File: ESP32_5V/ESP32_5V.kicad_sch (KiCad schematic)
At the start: 4 parts

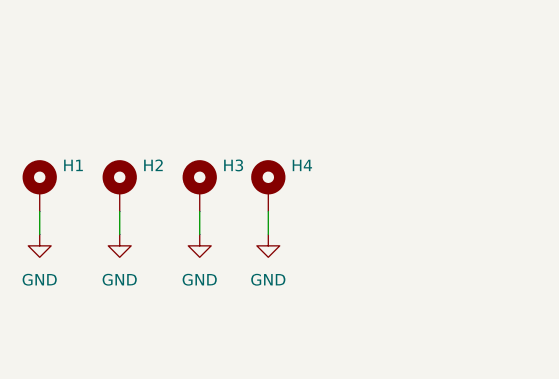
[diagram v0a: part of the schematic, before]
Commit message: update
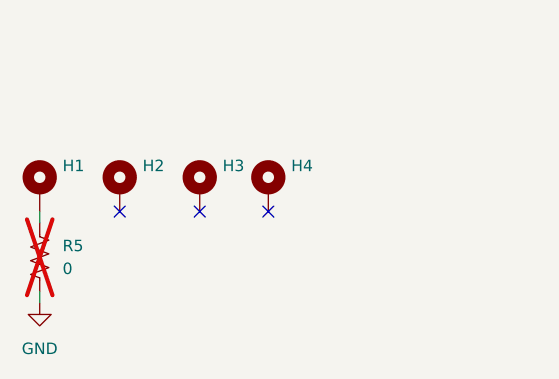
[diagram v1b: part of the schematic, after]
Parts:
- added R5: 0, symbol Device:R_US
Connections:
- net GND: now also R5.2; no longer H1.1, H2.1, H3.1, H4.1
- new net: H1.1, R5.1
- no-connect marks 0 -> 3
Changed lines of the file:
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@@
 		(color 0 0 0 0)
 	)
+	(no_connect
+		(at 57.15 177.8)
+	)
+	(no_connect
+		(at 40.64 177.8)
+	)
+	(no_connect
+		(at 49.53 177.8)
+	)
 	(wire
 		(pts
@@
 	(wire
 		(pts
-			(xy 31.75 180.34) (xy 31.75 177.8)
-		)
-		(stroke
-			(width 0)
-			(type default)
-		)
-	)
-	(wire
-		(pts
 			(xy 175.26 82.55) (xy 175.26 64.77)
 		)
@@
 	(wire
 		(pts
-			(xy 40.64 180.34) (xy 40.64 177.8)
-		)
-		(stroke
-			(width 0)
-			(type default)
-		)
-	)
-	(wire
-		(pts
 			(xy 185.42 127.635) (xy 185.42 62.23)
 		)
@@
 	(wire
 		(pts
+			(xy 31.75 187.96) (xy 31.75 186.69)
+		)
+		(stroke
+			(width 0)
+			(type default)
+		)
+	)
+	(wire
+		(pts
 			(xy 176.53 80.01) (xy 176.53 62.23)
 		)
@@
 	(wire
 		(pts
-			(xy 49.53 180.34) (xy 49.53 177.8)
-		)
-		(stroke
-			(width 0)
-			(type default)
-		)
-	)
-	(wire
-		(pts
 			(xy 139.065 97.155) (xy 170.18 97.155)
 		)
@@
 	(wire
 		(pts
-			(xy 57.15 180.34) (xy 57.15 177.8)
-		)
-		(stroke
-			(width 0)
-			(type default)
-		)
-	)
-	(wire
-		(pts
 			(xy 185.42 62.23) (xy 185.42 44.45)
 		)
@@
 		(pts
 			(xy 189.23 54.61) (xy 204.47 54.61)
+		)
+		(stroke
+			(width 0)
+			(type default)
+		)
+	)
+	(wire
+		(pts
+			(xy 31.75 179.07) (xy 31.75 177.8)
 		)
 		(stroke
@@
 	(symbol
 		(lib_id "power:GND")
-		(at 49.53 180.34 0)
-		(unit 1)
-		(exclude_from_sim no)
-		(in_bom yes)
-		(on_board yes)
-		(dnp no)
-		(fields_autoplaced yes)
-		(property "Reference" "#PWR033"
-			(at 49.53 186.69 0)
-			(effects
-				(font
-					(size 1.27 1.27)
-				)
-				(hide yes)
-			)
-		)
-		(property "Value" "GND"
-			(at 49.53 185.42 0)
-			(effects
-				(font
-					(size 1.27 1.27)
-				)
-			)
-		)
-		(property "Footprint" ""
-			(at 49.53 180.34 0)
-			(effects
-				(font
-					(size 1.27 1.27)
-				)
-				(hide yes)
-			)
-		)
-		(property "Datasheet" ""
-			(at 49.53 180.34 0)
-			(effects
-				(font
-					(size 1.27 1.27)
-				)
-				(hide yes)
-			)
-		)
-		(property "Description" "Power symbol creates a global label with name \"GND\" , ground"
-			(at 49.53 180.34 0)
-			(effects
-				(font
-					(size 1.27 1.27)
-				)
-				(hide yes)
-			)
-		)
-		(pin "1"
-		)
-		(instances
-			(project "ESP32_5V"
-				(path "/a7bda8b3-4b40-4c73-a9d2-e587ed8710cd"
-					(reference "#PWR033")
-					(unit 1)
-				)
-			)
-		)
-	)
-	(symbol
-		(lib_id "power:GND")
-		(at 31.75 180.34 0)
+		(at 31.75 187.96 0)
 		(unit 1)
 		(exclude_from_sim no)
@@
 		(fields_autoplaced yes)
 		(property "Reference" "#PWR031"
-			(at 31.75 186.69 0)
+			(at 31.75 194.31 0)
 			(effects
 				(font
@@
 		)
 		(property "Value" "GND"
-			(at 31.75 185.42 0)
+			(at 31.75 193.04 0)
 			(effects
 				(font
@@
 		)
 		(property "Footprint" ""
-			(at 31.75 180.34 0)
+			(at 31.75 187.96 0)
 			(effects
 				(font
@@
 		)
 		(property "Datasheet" ""
-			(at 31.75 180.34 0)
+			(at 31.75 187.96 0)
 			(effects
 				(font
@@
 		)
 		(property "Description" "Power symbol creates a global label with name \"GND\" , ground"
-			(at 31.75 180.34 0)
+			(at 31.75 187.96 0)
 			(effects
 				(font
@@
 	)
 	(symbol
-		(lib_id "power:GND")
-		(at 57.15 180.34 0)
+		(lib_id "Device:R_US")
+		(at 31.75 182.88 0)
 		(unit 1)
 		(exclude_from_sim no)
 		(in_bom yes)
 		(on_board yes)
-		(dnp no)
+		(dnp yes)
 		(fields_autoplaced yes)
-		(property "Reference" "#PWR034"
-			(at 57.15 186.69 0)
-			(effects
-				(font
-					(size 1.27 1.27)
-				)
-				(hide yes)
-			)
-		)
-		(property "Value" "GND"
-			(at 57.15 185.42 0)
-			(effects
-				(font
-					(size 1.27 1.27)
-				)
+		(property "Reference" "R5"
+			(at 34.29 181.6099 0)
+			(effects
+				(font
+					(size 1.27 1.27)
+				)
+				(justify left)
+			)
+		)
+		(property "Value" "0"
+			(at 34.29 184.1499 0)
+			(effects
+				(font
+					(size 1.27 1.27)
+				)
+				(justify left)
 			)
 		)
 		(property "Footprint" ""
-			(at 57.15 180.34 0)
-			(effects
-				(font
-					(size 1.27 1.27)
-				)
-				(hide yes)
-			)
-		)
-		(property "Datasheet" ""
-			(at 57.15 180.34 0)
-			(effects
-				(font
-					(size 1.27 1.27)
-				)
-				(hide yes)
-			)
-		)
-		(property "Description" "Power symbol creates a global label with name \"GND\" , ground"
-			(at 57.15 180.34 0)
-			(effects
-				(font
-					(size 1.27 1.27)
-				)
-				(hide yes)
-			)
+			(at 32.766 183.134 90)
+			(effects
+				(font
+					(size 1.27 1.27)
+				)
+				(hide yes)
+			)
+		)
+		(property "Datasheet" "~"
+			(at 31.75 182.88 0)
+			(effects
+				(font
+					(size 1.27 1.27)
+				)
+				(hide yes)
+			)
+		)
+		(property "Description" "Resistor, US symbol"
+			(at 31.75 182.88 0)
+			(effects
+				(font
+					(size 1.27 1.27)
+				)
+				(hide yes)
+			)
+		)
+		(pin "2"
 		)
 		(pin "1"
 		)
 		(instances
-			(project "ESP32_5V"
+			(project ""
 				(path "/a7bda8b3-4b40-4c73-a9d2-e587ed8710cd"
-					(reference "#PWR034")
+					(reference "R5")
 					(unit 1)
 				)
-			)
-		)
-	)
-	(symbol
-		(lib_id "power:GND")
-		(at 40.64 180.34 0)
-		(unit 1)
-		(exclude_from_sim no)
-		(in_bom yes)
-		(on_board yes)
-		(dnp no)
-		(fields_autoplaced yes)
-		(property "Reference" "#PWR032"
-			(at 40.64 186.69 0)
-			(effects
-				(font
-					(size 1.27 1.27)
-				)
-				(hide yes)
-			)
-		)
-		(property "Value" "GND"
-			(at 40.64 185.42 0)
-			(effects
-				(font
-					(size 1.27 1.27)
-				)
-			)
-		)
-		(property "Footprint" ""
-			(at 40.64 180.34 0)
-			(effects
-				(font
-					(size 1.27 1.27)
-				)
-				(hide yes)
-			)
-		)
-		(property "Datasheet" ""
-			(at 40.64 180.34 0)
-			(effects
-				(font
-					(size 1.27 1.27)
-				)
-				(hide yes)
-			)
-		)
-		(property "Description" "Power symbol creates a global label with name \"GND\" , ground"
-			(at 40.64 180.34 0)
-			(effects
-				(font
-					(size 1.27 1.27)
-				)
-				(hide yes)
-			)
-		)
-		(pin "1"
-		)
-		(instances
-			(project "ESP32_5V"
-				(path "/a7bda8b3-4b40-4c73-a9d2-e587ed8710cd"
-					(reference "#PWR032")
-					(unit 1)
-				)
